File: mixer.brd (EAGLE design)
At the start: 37 parts

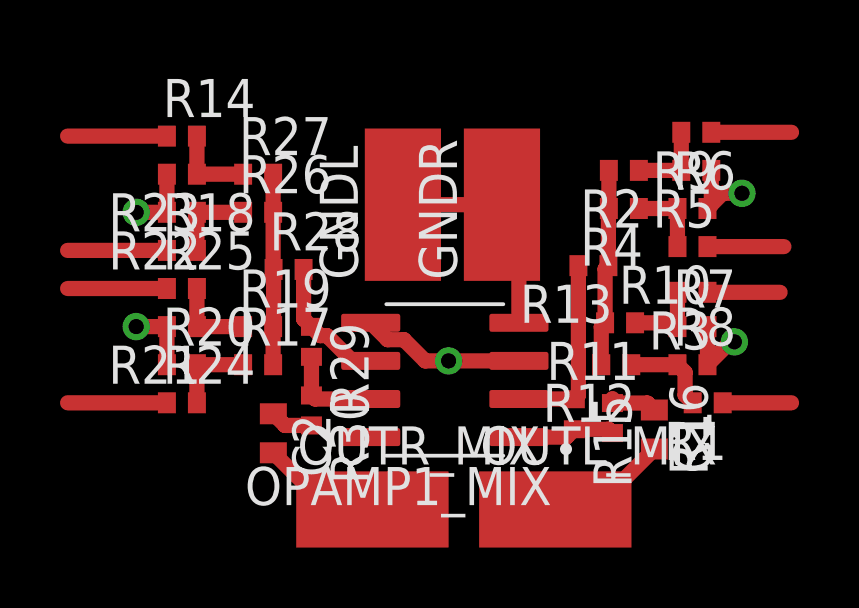
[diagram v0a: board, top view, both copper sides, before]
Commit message: v2 of board finished
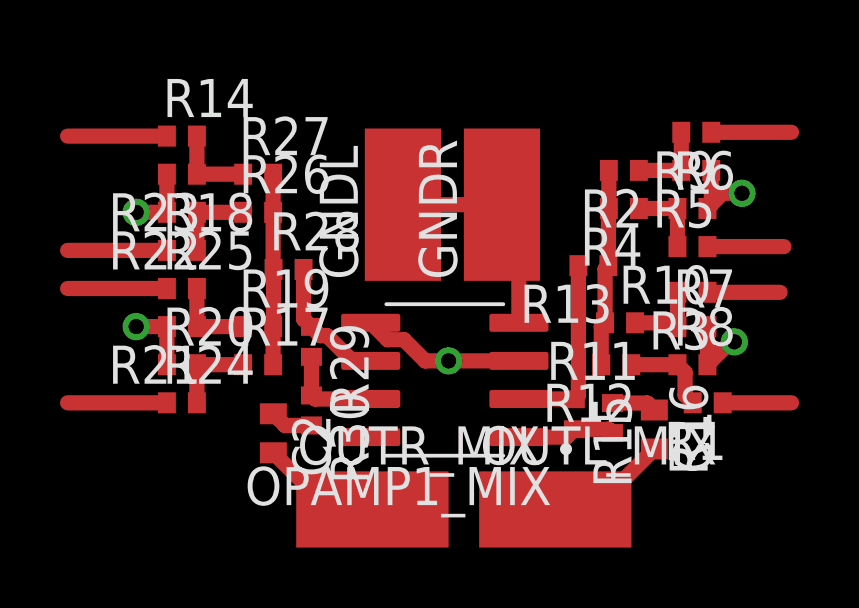
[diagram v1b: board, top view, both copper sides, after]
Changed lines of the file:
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@@
 <contactref element="R16" pad="2"/>
 <contactref element="C1" pad="1"/>
-<wire x1="13.081" y1="-8.748" x2="13.081" y2="-8.898" width="0.508" layer="1"/>
 <wire x1="13.081" y1="-8.898" x2="14.247" y2="-8.898" width="0.508" layer="1"/>
 <wire x1="14.247" y1="-8.898" x2="14.478" y2="-9.129" width="0.508" layer="1"/>
@@
 <wire x1="12.708" y1="-6.35" x2="12.835" y2="-6.223" width="0.508" layer="1"/>
 <wire x1="12.962" y1="-2.413" x2="12.962" y2="-1.143" width="0.508" layer="1"/>
-<wire x1="12.954" y1="-2.421" x2="12.962" y2="-2.413" width="0.508" layer="1"/>
-<wire x1="12.962" y1="-2.413" x2="12.946" y2="-2.429" width="0.508" layer="1"/>
-<wire x1="12.946" y1="-2.429" x2="12.946" y2="-4.318" width="0.508" layer="1"/>
 <wire x1="12.946" y1="-4.318" x2="12.835" y2="-4.429" width="0.508" layer="1"/>
 <wire x1="12.835" y1="-4.429" x2="12.835" y2="-6.223" width="0.508" layer="1"/>
+<wire x1="12.946" y1="-4.318" x2="12.946" y2="-2.429" width="0.508" layer="1"/>
+<wire x1="12.946" y1="-2.429" x2="12.962" y2="-2.413" width="0.508" layer="1"/>
 </signal>
 <signal name="N$15">
@@
 <contactref element="R13" pad="2"/>
 <contactref element="OPAMP1_MIX" pad="2"/>
-<wire x1="9.971" y1="-8.771" x2="9.963" y2="-8.763" width="0.508" layer="1"/>
 <wire x1="11.946" y1="-4.318" x2="11.946" y2="-8.636" width="0.508" layer="1"/>
-<wire x1="11.946" y1="-8.636" x2="11.811" y2="-8.771" width="0.508" layer="1"/>
-<wire x1="9.963" y1="-8.763" x2="11.803" y2="-8.763" width="0.508" layer="1"/>
+<wire x1="11.819" y1="-8.763" x2="11.811" y2="-8.771" width="0.508" layer="1"/>
 <wire x1="11.803" y1="-8.763" x2="11.811" y2="-8.771" width="0.508" layer="1"/>
+<wire x1="9.963" y1="-8.763" x2="11.819" y2="-8.763" width="0.508" layer="1"/>
+<wire x1="11.819" y1="-8.763" x2="11.946" y2="-8.636" width="0.508" layer="1"/>
 </signal>
 <signal name="OUT_A_MIX">
